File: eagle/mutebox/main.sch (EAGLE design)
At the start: 31 parts, among them IC1 6N138S-TA1, IC2 6N138S-TA1, SW1 RK09D1130C2P

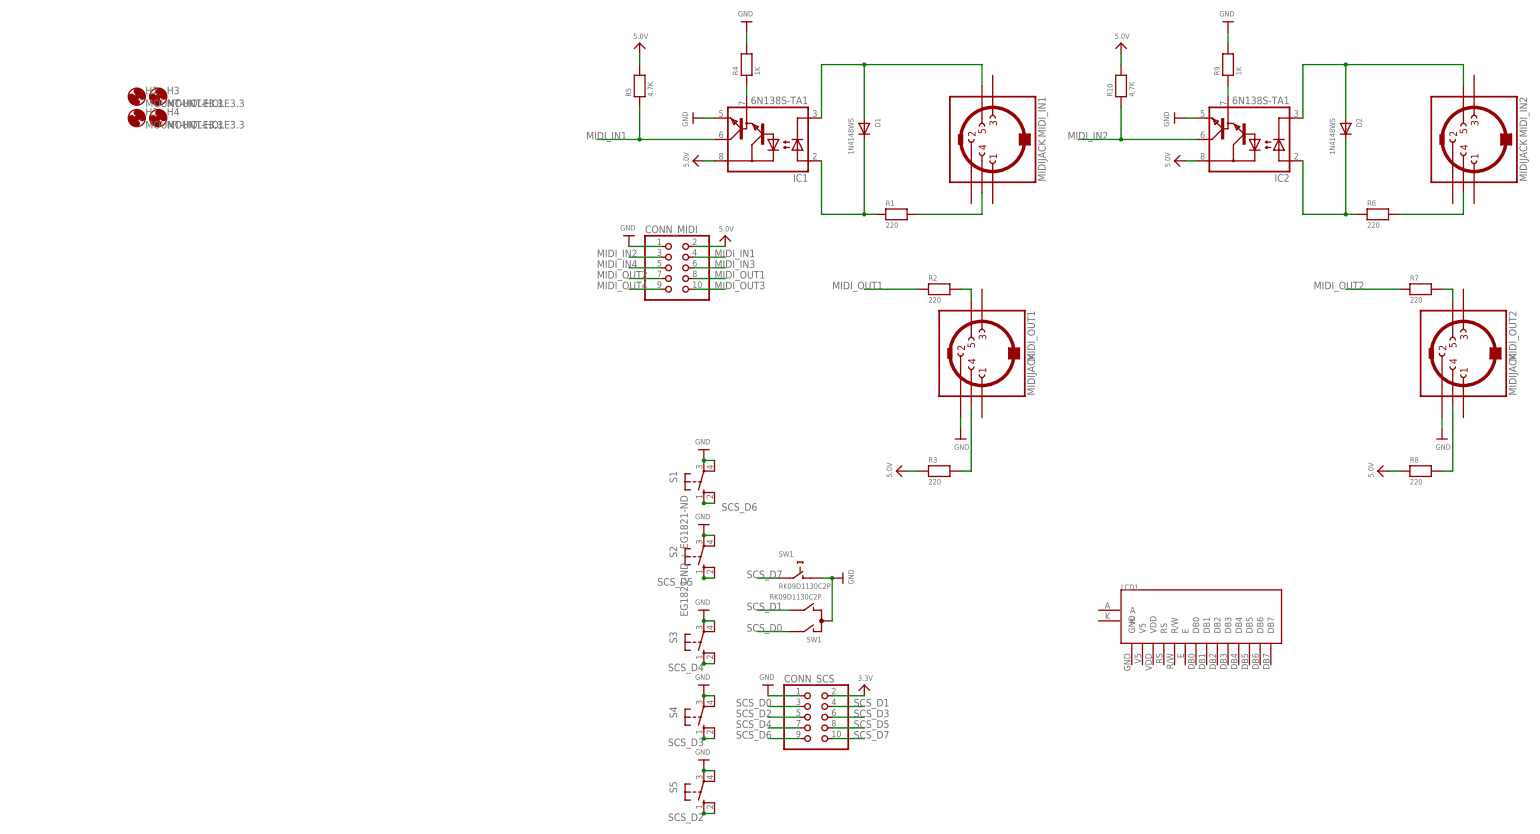
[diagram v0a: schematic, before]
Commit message: mutebox
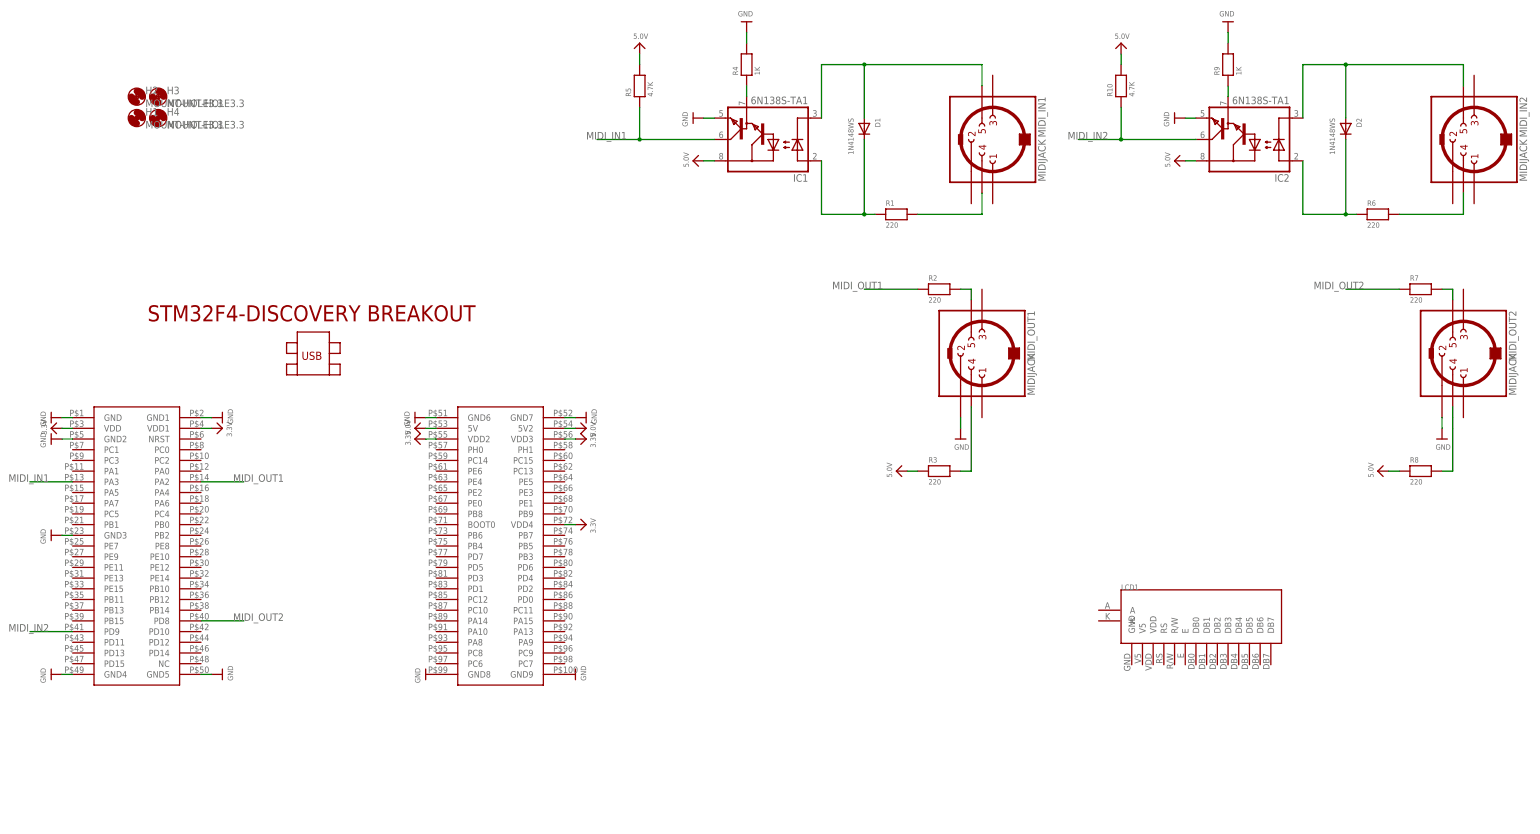
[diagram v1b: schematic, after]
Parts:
- removed CONN_MIDI, CONN_SCS: (no value), microbuilder:HEADER-2X5
- removed S1: EG1821-ND + EG1821-ND, og-switch:40-XX
- removed S2, S3, S4, S5: (no value), og-switch:40-XX
- removed SW1: RK09D1130C2P, switch-alps:EC12E_SW
- added U$1: STM32F4-DISCOVERY, STM32F4-DISCOVERY:STM32F4-DISCOVERY
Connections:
- removed net MIDI_IN3: CONN_MIDI.6
- removed net MIDI_IN4: CONN_MIDI.5
- removed net MIDI_OUT3: CONN_MIDI.10
- removed net MIDI_OUT4: CONN_MIDI.9
- removed net SCS_D0: CONN_SCS.3, SW1G$1.A
- removed net SCS_D1: CONN_SCS.4, SW1G$1.B
- removed net SCS_D2: CONN_SCS.5, S5.S, S5.S1
- removed net SCS_D3: CONN_SCS.6, S4.S, S4.S1
- removed net SCS_D4: CONN_SCS.7, S3.S, S3.S1
- removed net SCS_D5: CONN_SCS.8, S2.S, S2.S1
- removed net SCS_D6: CONN_SCS.9, S1.S, S1.S1
- removed net SCS_D7: CONN_SCS.10, SW1G$2.2
- net 3.3V: now also U$1.VDD, U$1.VDD1, U$1.VDD2, U$1.VDD3, U$1.VDD4; no longer CONN_SCS.2
- net 5.0V: now also U$1.5V, U$1.5V2; no longer CONN_MIDI.2
- net GND: now also U$1.GND, U$1.GND1, U$1.GND2, U$1.GND3, U$1.GND4, U$1.GND5, U$1.GND6, U$1.GND7, U$1.GND8, U$1.GND9; no longer CONN_MIDI.1, CONN_SCS.1, S1.P, S1.P1, S2.P, S2.P1, S3.P, S3.P1, S4.P, S4.P1, S5.P, S5.P1, SW1G$1.C, SW1G$2.1
- net MIDI_IN1: now also U$1.PA3; no longer CONN_MIDI.4
- net MIDI_IN2: now also U$1.PD9; no longer CONN_MIDI.3
- net MIDI_OUT1: now also U$1.PA2; no longer CONN_MIDI.8
- net MIDI_OUT2: now also U$1.PD8; no longer CONN_MIDI.7

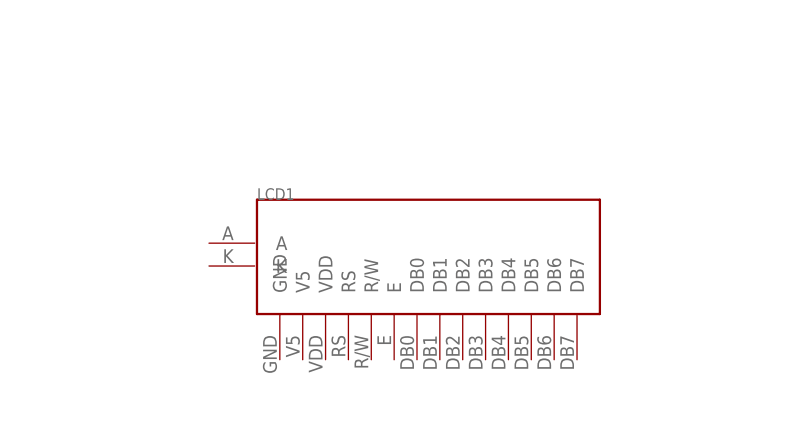
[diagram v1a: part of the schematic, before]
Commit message: wip
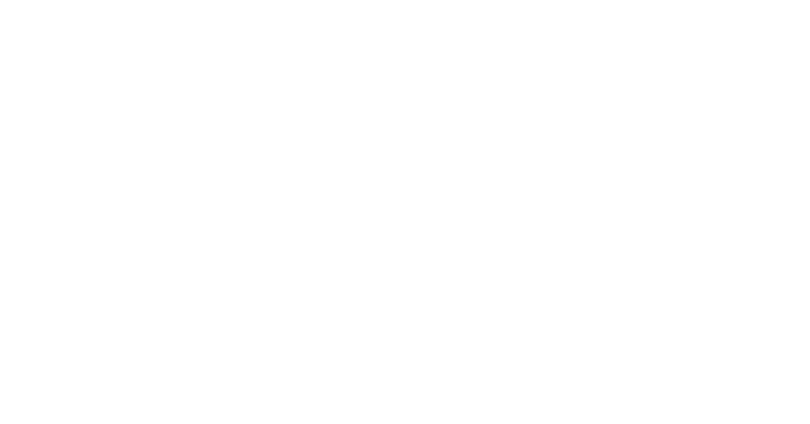
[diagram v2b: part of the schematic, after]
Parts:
- removed LCD1: NHD-C0220AA-FSW-FTW, NHD-C0220AA-FSW-FTW:NHD-C0220AA-FSW-FTW
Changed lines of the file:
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@@
 <part name="H3" library="holes" deviceset="MOUNT-HOLE" device="3.3"/>
 <part name="H4" library="holes" deviceset="MOUNT-HOLE" device="3.3"/>
-<part name="LCD1" library="NHD-C0220AA-FSW-FTW" deviceset="NHD-C0220AA-FSW-FTW" device=""/>
 </parts>
 <sheets>
@@
 <instance part="H3" gate="G$1" x="104.14" y="132.08"/>
 <instance part="H4" gate="G$1" x="104.14" y="127"/>
-<instance part="LCD1" gate="G$1" x="350.52" y="7.62"/>
 </instances>
 <busses>
